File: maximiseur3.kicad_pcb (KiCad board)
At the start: 2 copper layers, 150 x 100 mm, 45 parts, among them J1 PV+/M+, J2 M-, J3 PV-, P1 SW SW, Q1 IRLB3036G, Q2 IRLB3036G, Q3 IRLB3036G, Q4 IRLB3036G, T1 BD139, U1 LM311

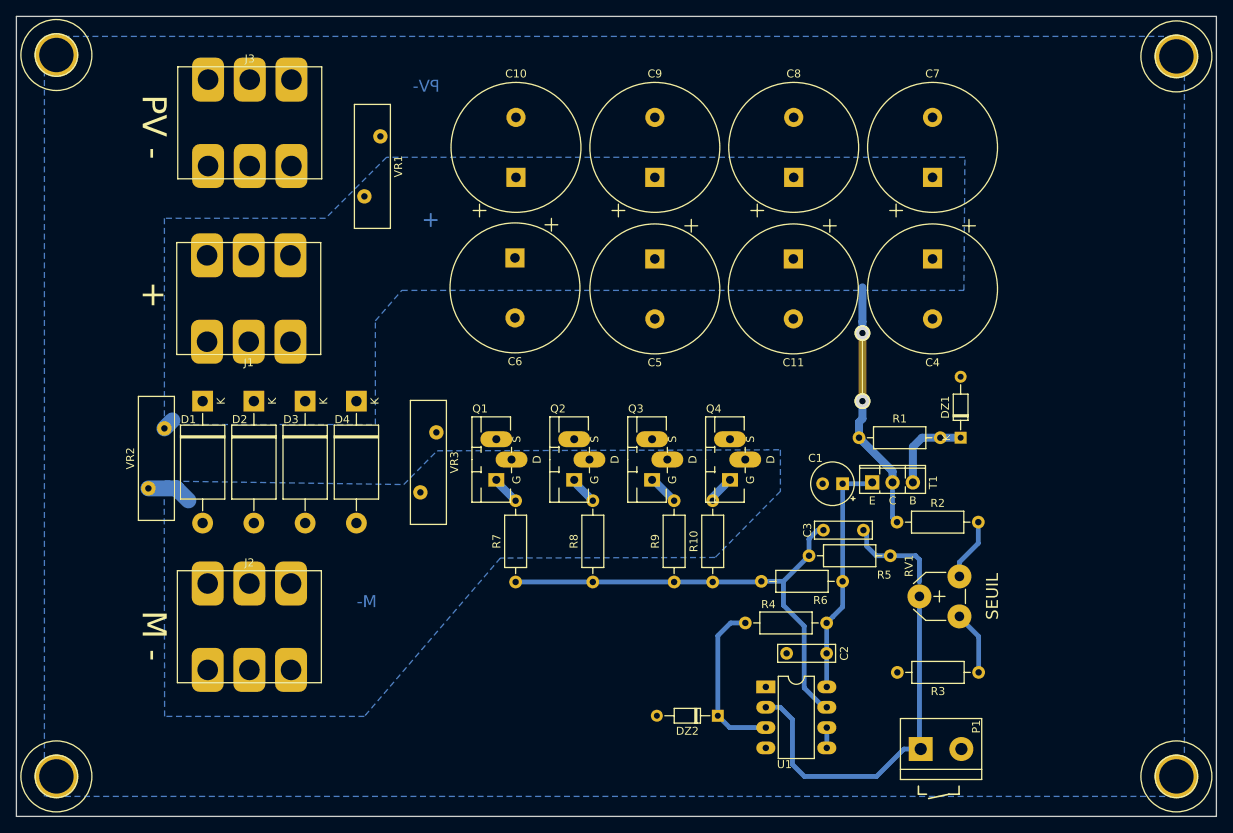
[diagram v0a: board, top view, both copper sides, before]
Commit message: derniers ajustements sur serigraphie avant export
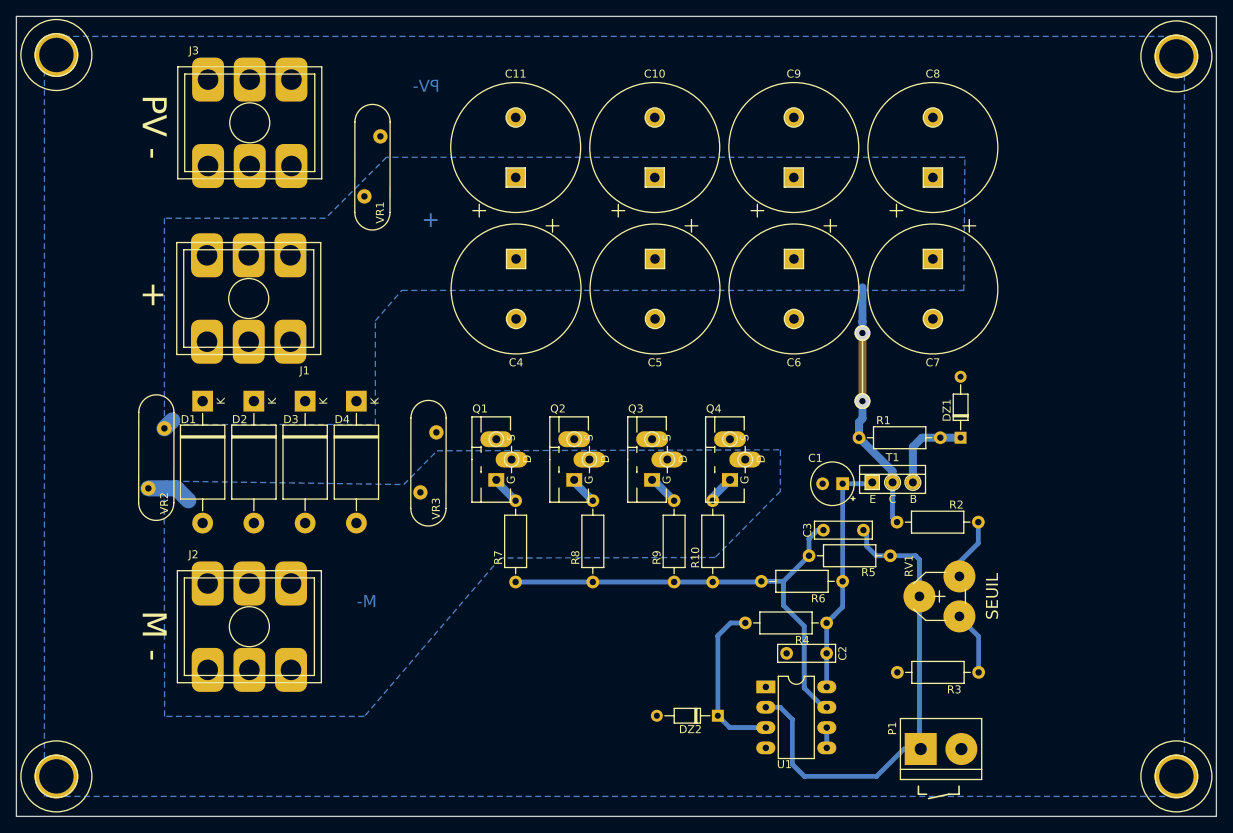
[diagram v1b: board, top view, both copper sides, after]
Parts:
- C1: footprint Capacitor_THT:CP_Radial_D5.0mm_P2.50mm -> maximiseur:CP_Radial_D5.0mm_P2.50mm
- C2, C3: footprint Capacitor_THT:C_Rect_L7.0mm_W2.0mm_P5.00mm -> maximiseur:C_Rect_L7.0mm_W2.0mm_P5.00mm
- DZ1: value 15V -> 12V; footprint Diode_THT:D_DO-34_SOD68_P7.62mm_Horizontal -> maximiseur:D_DO-34_SOD68_P7.62mm_Horizontal
- DZ2: footprint Diode_THT:D_DO-34_SOD68_P7.62mm_Horizontal -> maximiseur:D_DO-34_SOD68_P7.62mm_Horizontal
- R1, R10, R2, R3, R4, R5, R6, R7, R8, R9: footprint Resistor_THT:R_Axial_DIN0207_L6.3mm_D2.5mm_P10.16mm_Horizontal -> maximiseur:R_Axial_DIN0207_L6.3mm_D2.5mm_P10.16mm_Horizontal
- T1: footprint Package_TO_SOT_THT:TO-126-3_Vertical -> maximiseur:TO-126-3_Vertical
- U1: footprint Package_DIP:DIP-8_W7.62mm_LongPads -> maximiseur:DIP-8_W7.62mm_LongPads
- VR1, VR2, VR3: footprint Varistor:RV_Disc_D15.5mm_W4.5mm_P7.5mm -> maximiseur:RV_Disc_D15.5mm_W4.5mm_P7.5mm
- moved C4 52.1 mm to (99.0, 64.9)
- moved C11 36.2 mm to (99.0, 54.7), turned to 90 degrees
- moved C6 34.9 mm to (133.8, 64.9)
- moved C8 17.4 mm to (151.1, 54.7)
- moved C9 17.4 mm to (133.8, 54.7)
- moved C10 17.3 mm to (116.4, 54.7)
- moved C7 10.2 mm to (151.1, 64.9), turned to 270 degrees
